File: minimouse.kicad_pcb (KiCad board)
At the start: 2 copper layers, 90 x 85 mm, 54 parts, among them J1 Conn_ARM_JTAG_SWD_10, J4 Conn_01x06, J5 Conn_01x02, J6 Conn_01x04, J7 Conn_01x06, M1 N20_encoder, M2 N20_encoder, U1 STM32F030C8Tx, U2 STSPIN240, U3 LP5907MFX-1.2, U4 HC-SR04

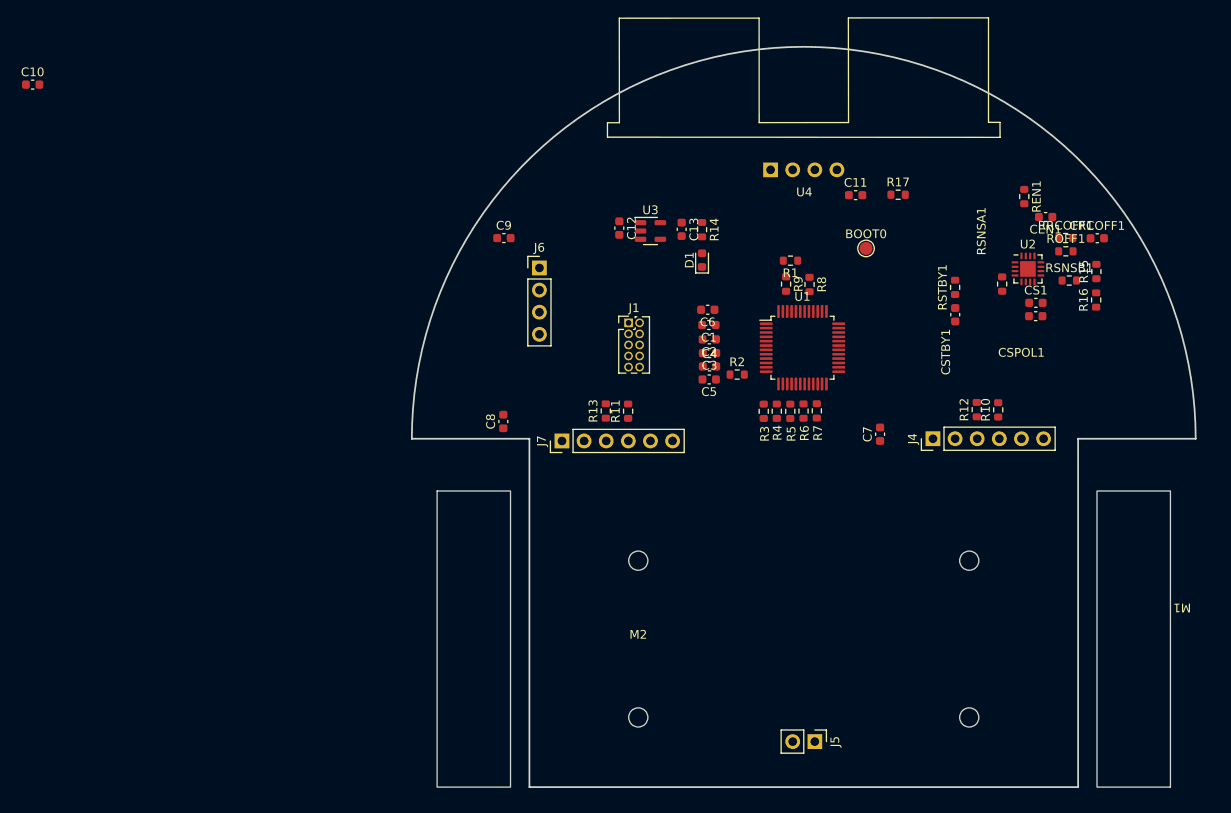
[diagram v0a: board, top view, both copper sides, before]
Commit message: nadjibmarouen
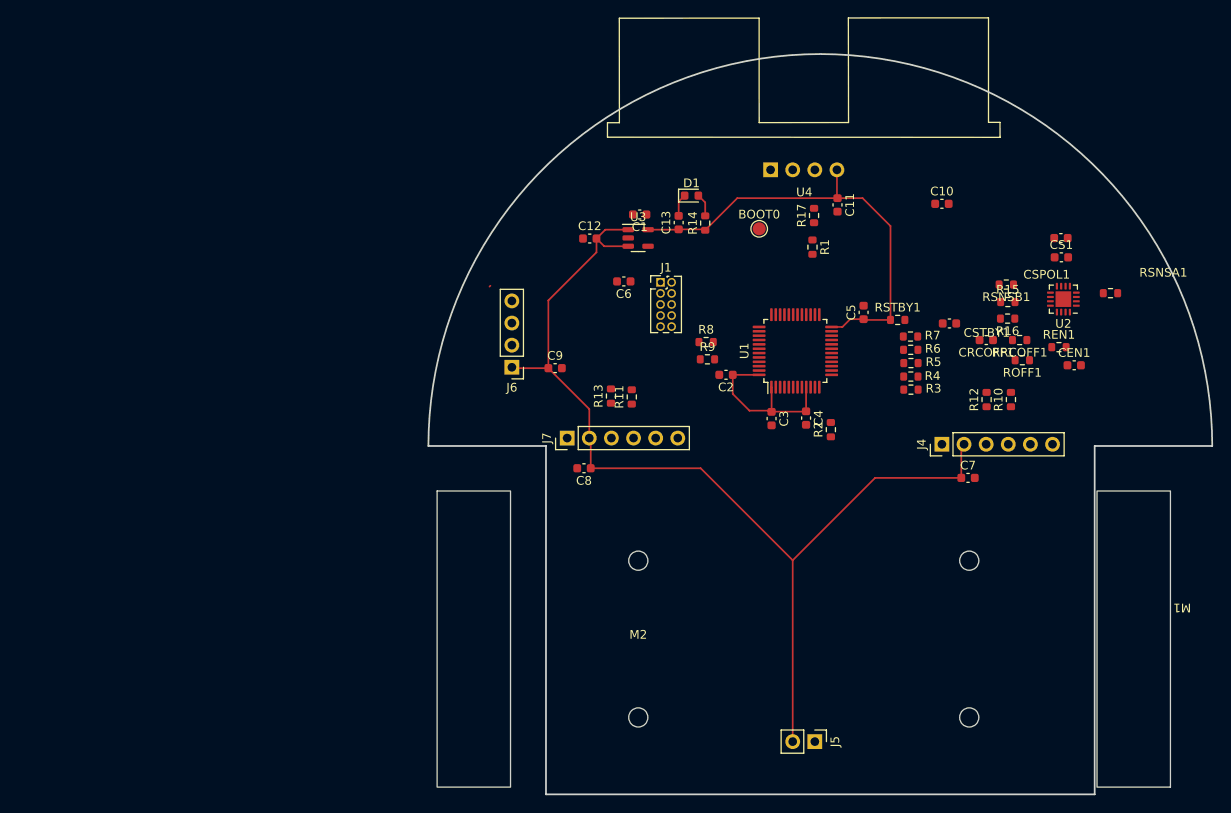
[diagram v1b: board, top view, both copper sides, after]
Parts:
- moved C10 105.3 mm to (165.9, 73.0)
- moved C5 19.3 mm to (156.9, 85.5), turned to 90 degrees
- moved REN1 17.7 mm to (179.3, 89.5), turned to 0 degrees
- moved CEN1 17.3 mm to (181.1, 91.6), turned to 0 degrees
- moved CRCOFF1 17.3 mm to (171.0, 88.7), turned to 180 degrees
- moved R3 17.1 mm to (162.3, 94.4), turned to 0 degrees
- moved C9 16.1 mm to (121.4, 91.9)
- moved R4 15.9 mm to (162.3, 92.9), turned to 0 degrees
- moved C1 15.0 mm to (131.2, 74.3)
- moved R5 14.9 mm to (162.3, 91.3), turned to 0 degrees
- moved R6 14.2 mm to (162.3, 89.8), turned to 180 degrees
- moved R7 13.7 mm to (162.3, 88.3), turned to 180 degrees
- moved R8 13.6 mm to (138.8, 88.9), turned to 0 degrees
- moved ROFF1 13.5 mm to (175.1, 91.0), turned to 180 degrees
- moved RRCOFF1 12.8 mm to (174.8, 88.7), turned to 180 degrees
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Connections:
- C12 pad 1: +BATT -> GND
- C12 pad 2: GND -> +BATT
- CS1 pad 1: +3.3V -> +BATT
- CSPOL1 pad 1: +3.3V -> +BATT
- U2 pad 6: +3.3V -> +BATT
- U4 pad 4: +BATT -> +3.3V
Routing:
- net +BATT: track 0.00 -> 119.4 mm
- net +3.3V: track 0.00 -> 72.2 mm
- net Net-(D1-A): track 0.00 -> 2.65 mm
- net GND: track 0.00 -> 2.61 mm
